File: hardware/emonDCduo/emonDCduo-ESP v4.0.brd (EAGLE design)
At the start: 114.2 x 76.5 mm, 106 parts, among them P1 B4B-PH-K, Y1 32Khz

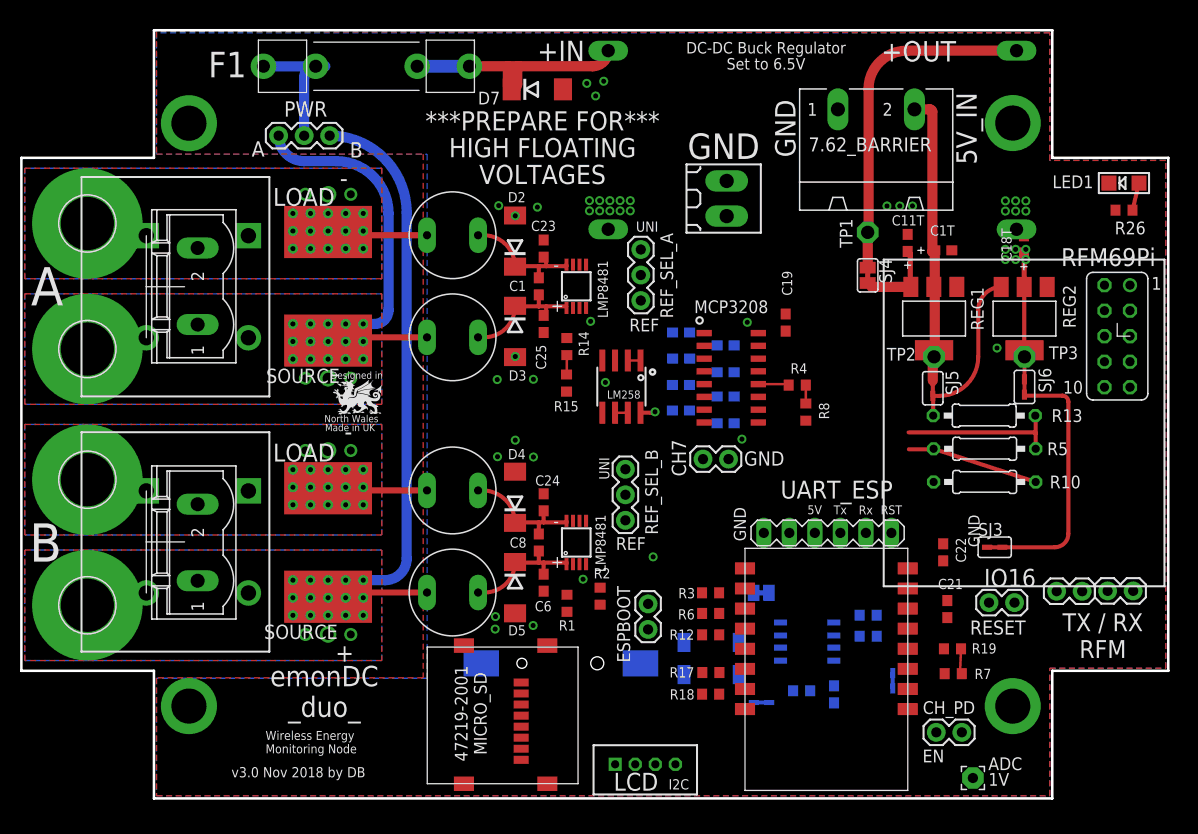
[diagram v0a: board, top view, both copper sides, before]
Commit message: commit v3.0
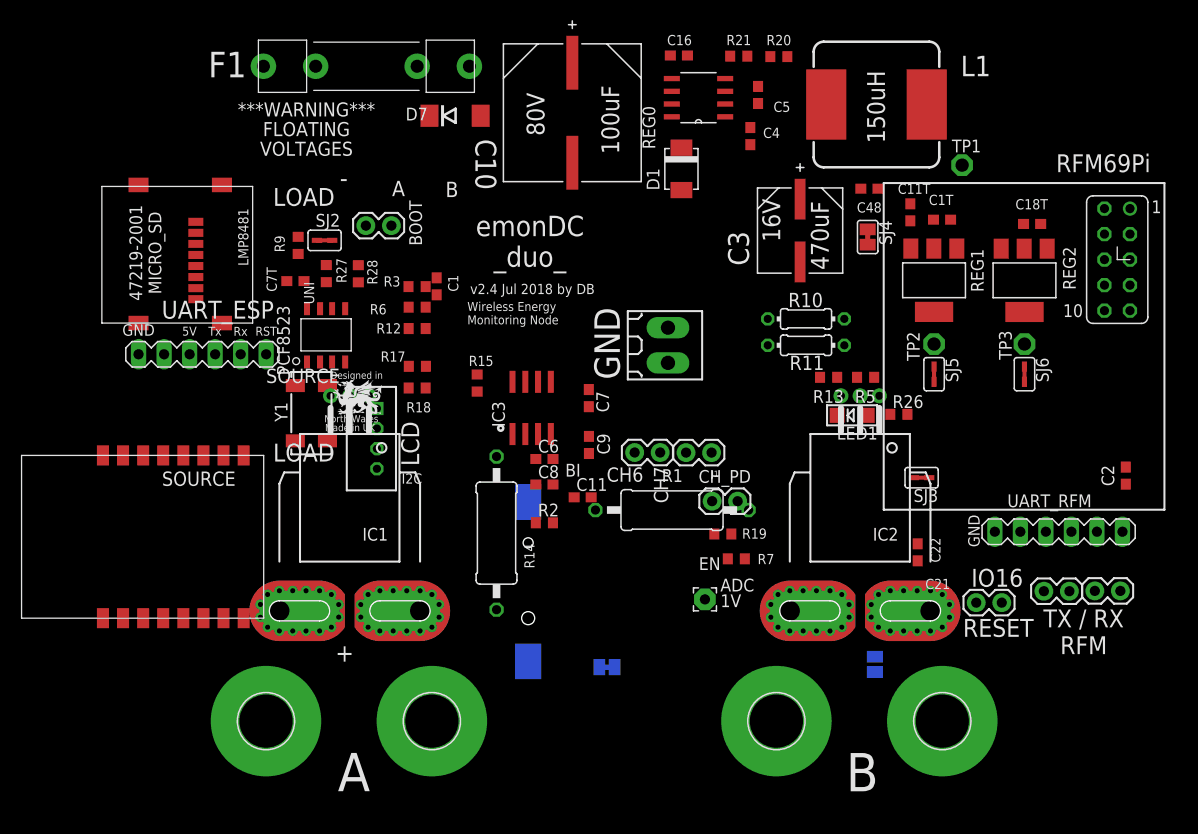
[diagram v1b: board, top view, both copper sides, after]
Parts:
- removed 7.62_BARRIER: GMSTBA2, con-phoenix-762:GMSTBA2
- removed C12, C13, C14, C15, C17, C18, C20: 1nF, rcl:C0603
- removed C19: 0.1uF, rcl:C0603
- removed C23, C24, C25: 0.1uF 100V, rcl:C0603
- removed D2, D3, D4, D5: P6SMB75A, diode:DO214AA
- removed EBW_A, EBW_B: EBW_SERIES_15.2MM, EBW series SHUNT:EBW_SERIES_15.2MM
- removed ESPBOOT: (no value), SparkFun:1X02
- removed F2, F3, F4, F5: (no value), fuse:TR5
- removed LM258: (no value), microbuilder:SOIC8_150MIL
- removed MCP3208: MCP3208-BI/SL, MCP3208:SOIC16
- removed MOUNT_10.16_A, MOUNT_10.16_B: MOLEX_39970-003, 10.16mm terminal block:2/10,16
- removed MOUNT_7.62_A, MOUNT_7.62_B: GMSTBV2, con-phoenix-762:GMSTBV2
- removed PWR, REF_SEL_A, REF_SEL_B: 455-1750-1-ND, SparkFun-Connectors:1X03
- removed R4: 1K, rcl:R0603
- removed R8: 2K, rcl:R0603
- removed SHUNTMON-A, SHUNTMON-B: LMP8481, lmp8481b:S-PDSO-G08
- removed SJ1: (no value), jumper-con_db:SJ-CON
- removed TP4, TP5, TP6, TP7: TPPAD1-13Y, testpad:P1-13Y
- added BOOT: (no value), SparkFun:1X02
- added C10: 100uF 80V, Panasonic-EEE-EEV-EEF-ECQ:CAPAE1350X1400N
- added C16: 0.1uF 100V, rcl:C0603
- added C2: 100nF, rcl:C0603
- added C3: 470uF 16V, Panasonic-EEEFK_EEEFP:CAPAE830X1050N
- added C4, C5: 0.1uF 16V, rcl:C0603
- added C48, C7, C9: 0.1uF, rcl:C0603
- added D1: MBRS1100T3G, diodes:SMB_1
- added IC1, IC2: ACS758LCB-050B-PFF-T, allegro:CB-PFF
- added IC3: LM358D, linear:SO08
- added J1: (no value), SparkFun-Connectors:1X02
- added L1: SRR1208, inductor-bourns:SSR1208
- added R11: 5.23k, rcl:0204/7
- added R20: 43k, rcl@1:R0603
- added R21: 10k, rcl@1:R0603
- added REG0: MAX5035, MAX5035:21-0111D_SBE-14
- added SJ7: (no value), jumper:SJ
- added UART_RFM: UART_RFM, JeeLabs:MA06-1
- C11: value 1nF -> 0.1uF 100V
- C11T, C18T, C1T: device rcl7:C0603POL -> rcl:C0603
- C7T: device rcl7:C0603POL -> rcl@1:C0603
- R1, R14: value 1M 100V -> 1.5M 3.5kV; device rcl:R0603 -> rcl7:0411/15
- R10: value 174R -> 16.56k; device rcl7:0207/10 -> rcl:0204/7
- R13: value 10k -> 5.23k; device rcl7:0207/10 -> rcl7:R0603
- R15, R2: value 56K -> 100K
- R26: value 174R -> 390R
- R5: value 5.6k -> 517.77k; device rcl7:0207/10 -> rcl7:R0603
- moved MH3 85.9 mm to (85.3, 9.47)
- moved MH4 72.7 mm to (68.8, 9.47)
- moved C7T 67.6 mm to (20.9, 53.3), flipped to the top, turned to 180 degrees
- moved R9 66.9 mm to (21.2, 56.8), flipped to the top, turned to 90 degrees
- moved R27 64.9 mm to (24.0, 54.0), flipped to the top, turned to 270 degrees
- moved UART_ESP 64.7 mm to (18.0, 46.0)
- moved ESP-12 64.5 mm to (17.8, 19.7), turned to 90 degrees
- moved SJ2 63.3 mm to (23.8, 57.3), flipped to the top
- moved R28 61.1 mm to (27.2, 54.0), flipped to the top, turned to 270 degrees
- moved PCF8523 56.7 mm to (24.0, 47.8), flipped to the top, turned to 90 degrees
- moved MICRO_SD 56.1 mm to (13.6, 49.1)
- moved MH2 52.6 mm to (18.0, 9.47)
- moved MH1 50.5 mm to (34.5, 9.47)
- moved Y1 46.7 mm to (22.5, 40.1), flipped to the top, turned to 270 degrees
- moved R12 42.2 mm to (33.1, 48.5)
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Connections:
- net RESET renamed N$30
- net VDD_PCF renamed N$10
- removed net GPIO12A: MCP3208.12, R4.1
- removed net LOAD-NEG-A_T: C1.1, C23.2, D2.C, F2.2, SHUNTMON-A.8
- removed net LOAD-NEG-B: EBW_A.P$18, EBW_A.P$19, EBW_A.P$2, EBW_A.P$20, EBW_A.P$21, EBW_A.P$22, EBW_A.P$23, EBW_A.P$24, EBW_A.P$25, EBW_A.P$26, EBW_A.P$27, EBW_A.P$28, EBW_A.P$29, EBW_A.P$30, EBW_A.P$31, EBW_A.P$32, EBW_A.P$36, EBW_A.P$37, EBW_A.P$38, F4.1, MH4.B5,5, MOUNT_10.16_B.P$1, MOUNT_10.16_B.P$2, MOUNT_7.62_A.2
- removed net LOAD-NEG-B_T: C24.2, C8.1, D4.C, F4.2, SHUNTMON-B.8
- removed net REF_A_INPUT: REF_SEL_A.2, SHUNTMON-A.6, SHUNTMON-A.7
- removed net REF_B_INPUT: REF_SEL_B.2, SHUNTMON-B.6, SHUNTMON-B.7
- removed net SOURCE-POS-A_T: C1.2, C25.1, D3.C, F3.2, R14.2, SHUNTMON-A.1
- removed net SOURCE-POS-B_T: C6.1, C8.2, D5.C, F5.2, R1.2, SHUNTMON-B.1
- removed net VSENSE_B: LM258.5, R1.1, R2.2
- new net BST: C4.1, REG0.1
- new net CH6: J5.2
- new net LX: C4.2, D1.C, L1.1, REG0.8
- new net N$20: UART_RFM.5
- new net N$3: IC2.IP+, IC2.IP+@10, IC2.IP+@11, IC2.IP+@12, IC2.IP+@13, IC2.IP+@14, IC2.IP+@15, IC2.IP+@16, IC2.IP+@17, IC2.IP+@2, IC2.IP+@3, IC2.IP+@4, IC2.IP+@5, IC2.IP+@6, IC2.IP+@7, IC2.IP+@8, IC2.IP+@9, MH4.B5,5
- new net N$301: C2.2, UART_RFM.1
- new net N$4: J1.2
- new net N$6: J1.1
- new net N$9: IC3.5, R1.1, R2.2
- new net PRE_6.5V: C3.1, C48.1, L1.2, R20.2, SJ4.1, TP1.TP
- new net V+: IC3.8
- new net V-: IC3.4
- new net VD: C5.1, REG0.2
- net +3V3: no longer C18.1, MCP3208.7
- net +5V: now also C1.1, C8.1, IC1.1, IC2.1, R10.2, R5.1, UART_RFM.4; no longer C19.1, LM258.8, MCP3208.15, MCP3208.16, R13.2, SHUNTMON-A.2, SHUNTMON-B.2
- net 5V_PRE: no longer 7.62_BARRIER.2
- net ADCSHUNT_A: now also C6.1, IC1.3; no longer C17.1, MCP3208.1, SHUNTMON-A.5
- net ADCSHUNT_B: now also C11.1, IC2.3; no longer C12.1, MCP3208.3, SHUNTMON-B.5
- net BI_REF: now also C7.1, R10.1, R11.2; no longer C14.1, MCP3208.5, R13.1, R5.2, REF_SEL_A.3, REF_SEL_B.3
- net CH7: no longer C20.1, MCP3208.8
- net D0/RX: now also UART_RFM.2
- net D1/TX: now also UART_RFM.3
- net GND: now also BOOT.1, C1.2, C10.2, C11.2, C16.2, C3.2, C48.2, C5.2, C7.2, C8.2, C9.2, D1.A, IC1.2, IC2.2, R11.1, R13.2, R21.1, REG0.3, REG0.6, UART_RFM.6; no longer 7.62_BARRIER.1, C19.2, C23.1, C24.1, C25.2, D2.A, D3.A, D4.A, D5.A, ESPBOOT.1, J5.2, LM258.4, MCP3208.14, MCP3208.9, R10.1, R8.2, SHUNTMON-A.4, SHUNTMON-B.4, TP6.TP, TP7.TP
- net GPIO0: now also BOOT.2; no longer ESPBOOT.2
- net GPIO12: no longer R4.2, R8.1
- net GPIO13: no longer MCP3208.11
- net GPIO14: no longer MCP3208.13
- net GPIO16: now also SJ7.1; no longer SJ1.2
- net GPIO2: no longer MCP3208.10
- net LOAD-NEG-A: now also IC1.IP+, IC1.IP+@10, IC1.IP+@11, IC1.IP+@12, IC1.IP+@13, IC1.IP+@14, IC1.IP+@15, IC1.IP+@16, IC1.IP+@17, IC1.IP+@2, IC1.IP+@3, IC1.IP+@4, IC1.IP+@5, IC1.IP+@6, IC1.IP+@7, IC1.IP+@8, IC1.IP+@9; no longer EBW_B.P$18, EBW_B.P$19, EBW_B.P$2, EBW_B.P$20, EBW_B.P$21, EBW_B.P$22, EBW_B.P$23, EBW_B.P$24, EBW_B.P$25, EBW_B.P$26, EBW_B.P$27, EBW_B.P$28, EBW_B.P$29, EBW_B.P$30, EBW_B.P$31, EBW_B.P$32, EBW_B.P$36, EBW_B.P$37, EBW_B.P$38, F2.1, MOUNT_10.16_A.P$1, MOUNT_10.16_A.P$2, MOUNT_7.62_B.2
- net N$1: now also R20.1, R21.2, REG0.4; no longer SJ4.1, TP1.TP, TP5.TP
- net RST: now also SJ7.2; no longer SJ1.1
- net SOURCE-POS-A: now also IC1.IP-, IC1.IP-@10, IC1.IP-@11, IC1.IP-@12, IC1.IP-@13, IC1.IP-@14, IC1.IP-@15, IC1.IP-@16, IC1.IP-@17, IC1.IP-@2, IC1.IP-@3, IC1.IP-@4, IC1.IP-@5, IC1.IP-@6, IC1.IP-@7, IC1.IP-@8, IC1.IP-@9, R14.2; no longer EBW_B.P$1, EBW_B.P$10, EBW_B.P$11, EBW_B.P$12, EBW_B.P$13, EBW_B.P$14, EBW_B.P$15, EBW_B.P$16, EBW_B.P$17, EBW_B.P$3, EBW_B.P$33, EBW_B.P$34, EBW_B.P$35, EBW_B.P$4, EBW_B.P$5, EBW_B.P$6, EBW_B.P$7, EBW_B.P$8, EBW_B.P$9, F3.1, MOUNT_10.16_A.P$3, MOUNT_10.16_A.P$4, MOUNT_7.62_B.1, PWR.3
- net SOURCE-POS-B: now also IC2.IP-, IC2.IP-@10, IC2.IP-@11, IC2.IP-@12, IC2.IP-@13, IC2.IP-@14, IC2.IP-@15, IC2.IP-@16, IC2.IP-@17, IC2.IP-@2, IC2.IP-@3, IC2.IP-@4, IC2.IP-@5, IC2.IP-@6, IC2.IP-@7, IC2.IP-@8, IC2.IP-@9, R1.2; no longer EBW_A.P$1, EBW_A.P$10, EBW_A.P$11, EBW_A.P$12, EBW_A.P$13, EBW_A.P$14, EBW_A.P$15, EBW_A.P$16, EBW_A.P$17, EBW_A.P$3, EBW_A.P$33, EBW_A.P$34, EBW_A.P$35, EBW_A.P$4, EBW_A.P$5, EBW_A.P$6, EBW_A.P$7, EBW_A.P$8, EBW_A.P$9, F5.1, MOUNT_10.16_B.P$3, MOUNT_10.16_B.P$4, MOUNT_7.62_A.1, PWR.1
- net UNI_REF: now also C9.1, R13.1, R5.2; no longer C15.1, MCP3208.6, R10.2, R5.1, REF_SEL_A.1, REF_SEL_B.1
- net VSENSE_A: now also IC3.3; no longer LM258.3
- net VSENSE_A_BUFF: now also IC3.1, IC3.2; no longer C11.1, LM258.1, LM258.2, MCP3208.2
- net VSENSE_B_BUFF: now also IC3.6, IC3.7; no longer C13.1, LM258.6, LM258.7, MCP3208.4
- net V_IN_POSTFUSE: now also C10.1, C16.1, REG0.5, REG0.7; no longer TP4.TP
- net V_IN_PREFUSE: no longer PWR.2
- net _RESET: now also C2.1
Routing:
- net SOURCE-POS-B: track 59.1 -> 0.00 mm
- net 5V_PRE: track 43.2 -> 0.00 mm
- net SOURCE-POS-A: track 37.4 -> 0.00 mm
- net N$1: track 34.1 -> 0.00 mm
- net V_IN_POSTFUSE: track 27.2 -> 0.00 mm
- net +3V3: track 24.9 -> 0.00 mm, vias 1 -> 0
- net +5V: track 17.6 -> 0.00 mm, vias 1 -> 0
- net BI_REF: track 16.1 -> 0.00 mm
- net LOAD-NEG-B_T: track 14.1 -> 0.00 mm
- net V_IN_PREFUSE: track 13.5 -> 0.00 mm
- net SOURCE-POS-B_T: track 13.2 -> 0.00 mm
- net UNI_REF: track 13.2 -> 0.00 mm
- net LOAD-NEG-A_T: track 12.6 -> 0.00 mm
- net 3.3V_PRE: track 12.6 -> 0.00 mm
- net SOURCE-POS-A_T: track 12.4 -> 0.00 mm
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- removed copper zone on layer 1, net GND
- removed copper zone on layer 16, net GND
- removed copper zone on layer 1, net LOAD-NEG-A
- removed copper zone on layer 16, net LOAD-NEG-A
- removed copper zone on layer 1, net LOAD-NEG-B
- removed copper zone on layer 16, net LOAD-NEG-B
- removed copper zone on layer 1, net SOURCE-POS-A
- removed copper zone on layer 16, net SOURCE-POS-A
- removed copper zone on layer 1, net SOURCE-POS-B
- removed copper zone on layer 16, net SOURCE-POS-B
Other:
- board size 114.2 x 76.5 mm -> 16 x 2 mm
- board text added: "***WARNING*** FLOATING VOLTAGES"
- board text added: "100uF"
- board text added: "150uH"
- board text added: "16V"
- board text added: "470uF"
- board text added: "80V"
- board text added: "BI"
- board text added: "CH6"
- board text added: "v2.4 Jul 2018 by DB"
- board text removed: "***PREPARE FOR*** HIGH FLOATING VOLTAGES"
- board text removed: "+IN"
- board text removed: "+OUT"
- board text removed: "5V_IN"
- board text removed: "DC-DC Buck Regulator Set to 6.5V"
- board text removed: "REF"
- board text removed: "v3.0 Nov 2018 by DB"
